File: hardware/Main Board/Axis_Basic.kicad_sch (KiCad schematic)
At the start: 58 parts, among them J1 USB_C_Receptacle_USB2.0, J2 JST_PH, J3 JST_PH, J4 S2B-PH-K-S, J5 1175-1628-ND, J6 1-84952-4, SW1 RKB2SJK, SW2 RKB2SJK, U1 TLV493D, U2 UA78M33CDCYR, U3 ATSAMD51G18A-MU, U4 TMC2209-LA, U5 AT25040B-MAHL-T, Y1 SG-210STF 48.0000ML0

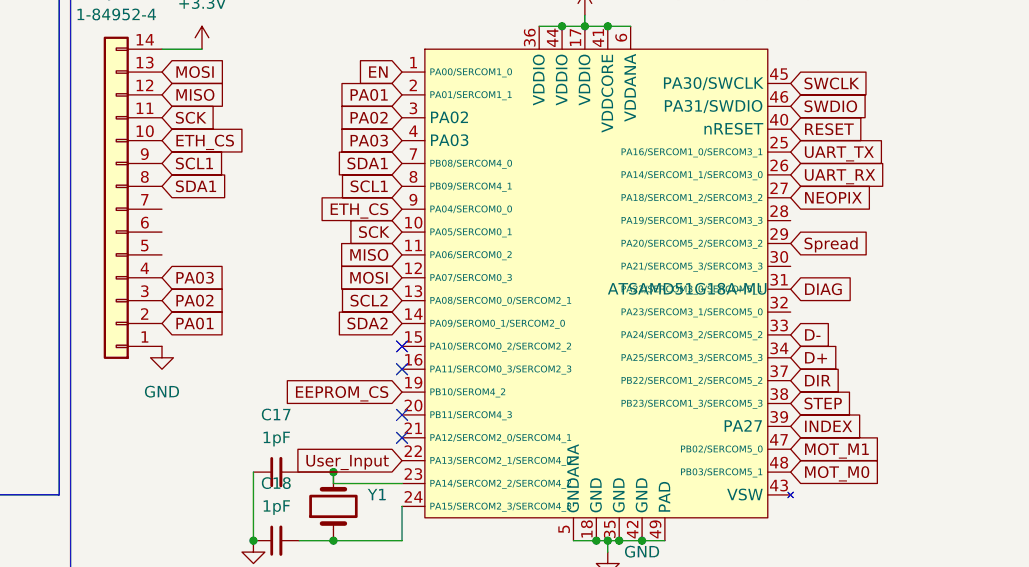
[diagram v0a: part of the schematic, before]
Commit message: PCB ordered
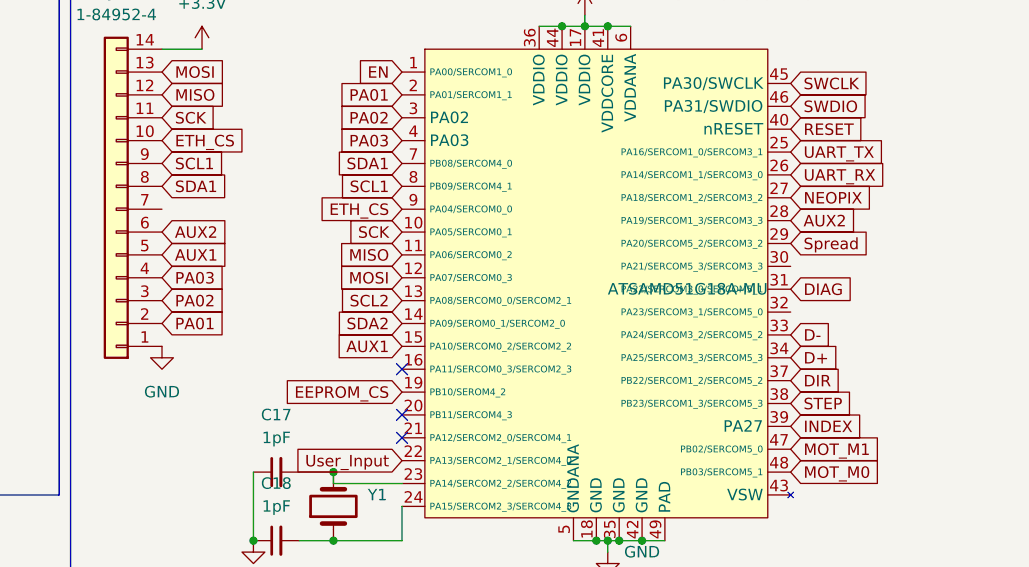
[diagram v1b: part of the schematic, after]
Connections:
- net AUX1: now reaches J6.5 (Pin_5)
- net AUX1: now also U3.15 (PA10/SERCOM0_2/SERCOM2_2)
- net AUX2: now reaches J6.6 (Pin_6)
- net AUX2: now also U3.28 (PA19/SERCOM1_3/SERCOM3_3)
- no-connect marks 11 -> 10
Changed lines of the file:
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@@
   (no_connect (at 40.64 54.61))
   (no_connect (at 139.7 39.37))
-  (no_connect (at 90.17 128.27))
   (no_connect (at 33.02 110.49))
   (no_connect (at 196.85 139.7))
@@
     )
   )
+  (global_label "AUX2" (shape input) (at 133.35 114.3 0) (fields_autoplaced)
+    (effects (font (size 1.27 1.27)) (justify left))
+    (property "Intersheetrefs" "${INTERSHEET_REFS}" (at 141.1733 114.3 0)
+      (effects (font (size 1.27 1.27)) (justify left) hide)
+    )
+  )
   (global_label "MOTOR_B2" (shape input) (at 237.49 121.92 0) (fields_autoplaced)
     (effects (font (size 1.27 1.27)) (justify left))
@@
     )
   )
+  (global_label "AUX2" (shape input) (at 63.5 115.57 0) (fields_autoplaced)
+    (effects (font (size 1.27 1.27)) (justify left))
+    (property "Intersheetrefs" "${INTERSHEET_REFS}" (at 71.3233 115.57 0)
+      (effects (font (size 1.27 1.27)) (justify left) hide)
+    )
+  )
   (global_label "EN" (shape input) (at 196.85 101.6 180) (fields_autoplaced)
     (effects (font (size 1.27 1.27)) (justify right))
@@
     )
   )
+  (global_label "AUX1" (shape input) (at 90.17 128.27 180) (fields_autoplaced)
+    (effects (font (size 1.27 1.27)) (justify right))
+    (property "Intersheetrefs" "${INTERSHEET_REFS}" (at 82.3467 128.27 0)
+      (effects (font (size 1.27 1.27)) (justify right) hide)
+    )
+  )
   (global_label "DIR" (shape input) (at 133.35 132.08 0) (fields_autoplaced)
     (effects (font (size 1.27 1.27)) (justify left))
@@
       (effects (font (size 1.27 1.27)) (justify left) hide)
     )
+  )
+  (global_label "AUX1" (shape input) (at 63.5 118.11 0) (fields_autoplaced)
+    (effects (font (size 1.27 1.27)) (justify left))
+    (property "Intersheetrefs" "${INTERSHEET_REFS}" (at 71.3233 118.11 0)
+      (effects (font (size 1.27 1.27)) (justify left) hide)
+    )
